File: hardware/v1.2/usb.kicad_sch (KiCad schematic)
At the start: 45 parts, among them J3 USB_C_Receptacle_USB2.0_14P, J4 USB_C_Receptacle_USB2.0_14P, J5 USB_C_Receptacle_USB2.0_14P, U1 ECP5U_25F_CABGA256, U6 FT231XQ, U7 TPD2EUSB30A, U8 TPD2EUSB30A, U9 TPD2EUSB30A

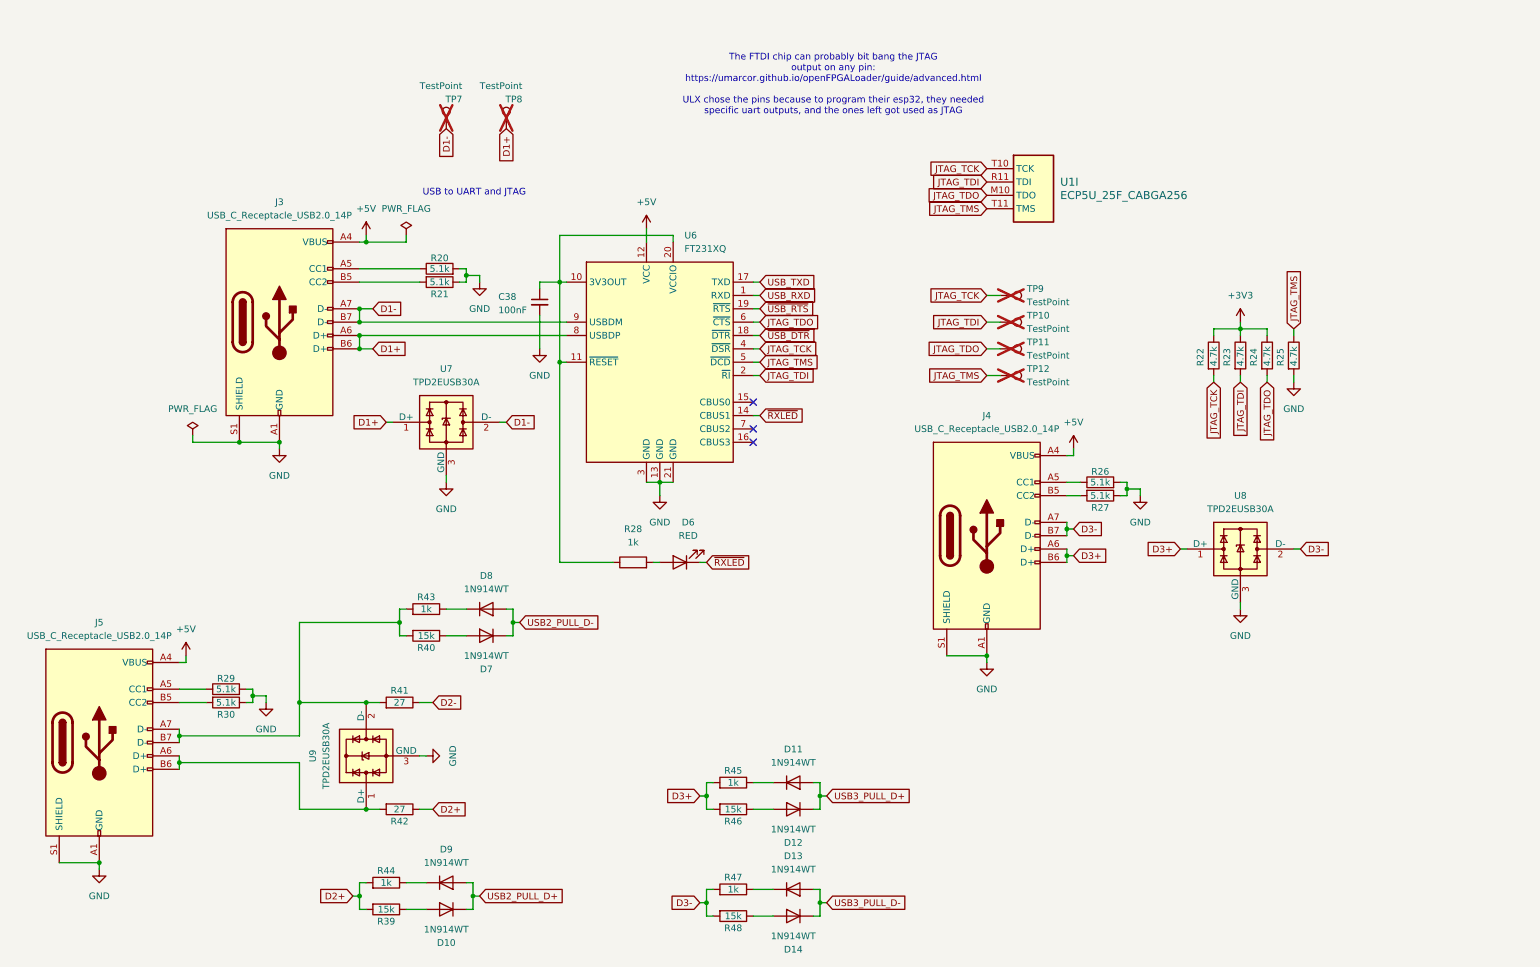
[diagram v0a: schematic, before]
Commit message: Trying to document my journey :)
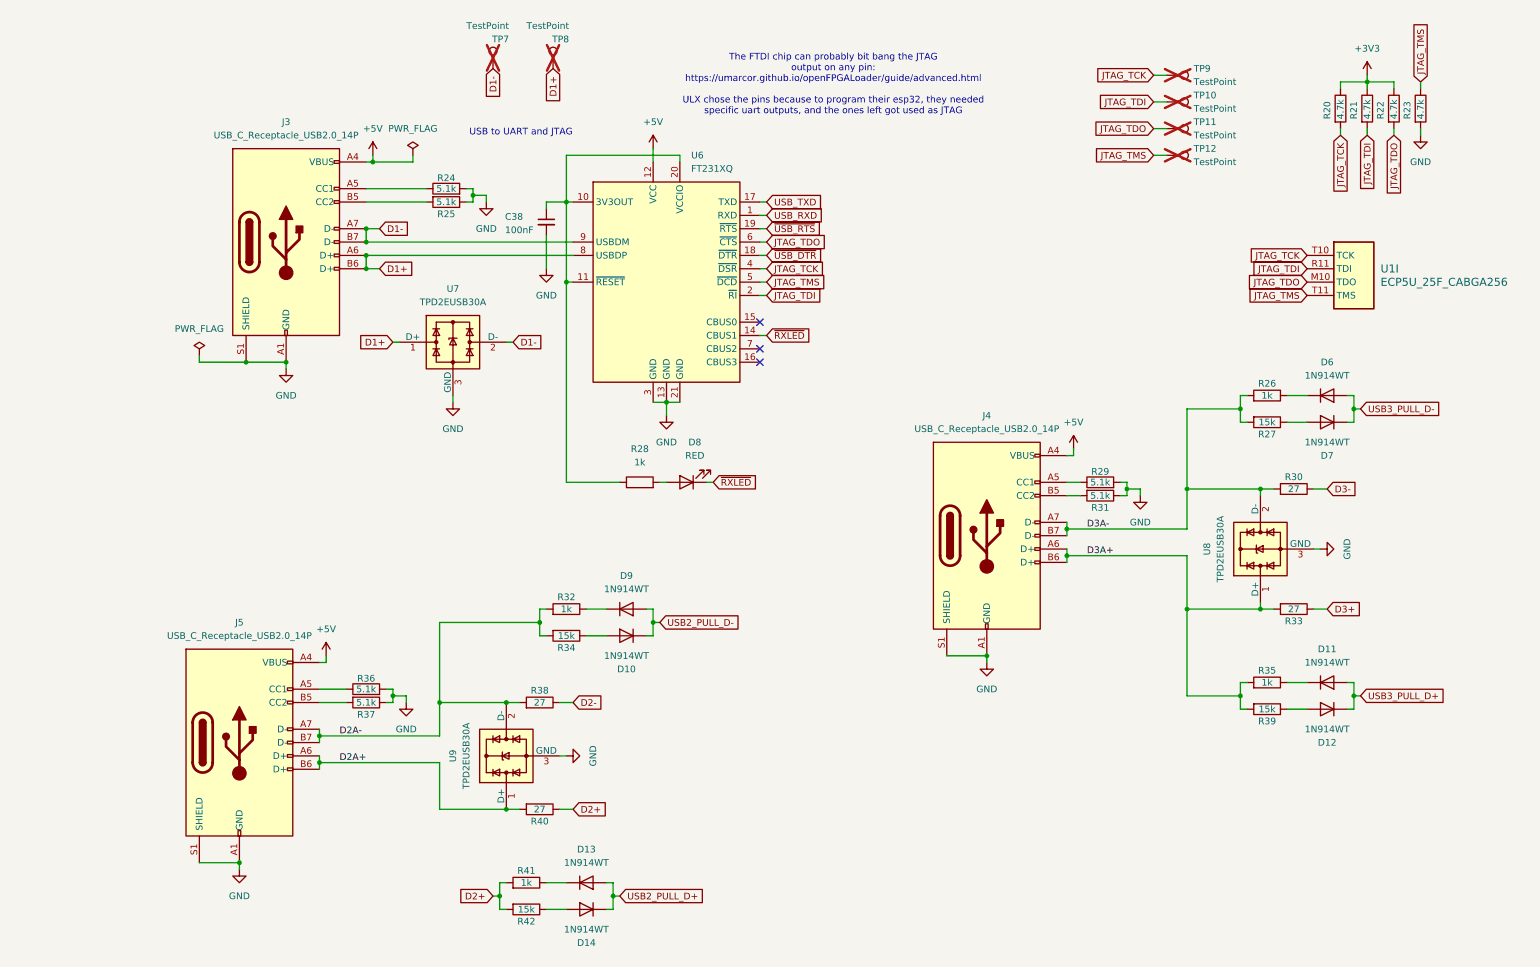
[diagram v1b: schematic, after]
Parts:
- added R30, R33: 27, Resistor_SMD:R_0201_0603Metric, symbol Device:R
- renumbered D7 to D10, D9 to D13, D10 to D14, D13 to D6, D14 to D7, D6 to D8, D8 to D9, R22 to R20, R23 to R21, R24 to R22, R25 to R23, R20 to R24, R21 to R25, R47 to R26, R48 to R27, R26 to R29, R27 to R31, R43 to R32, R40 to R34, R45 to R35, R29 to R36, R30 to R37, R41 to R38, R46 to R39, R42 to R40, R44 to R41, R39 to R42
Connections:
- net D3+: now also R33.1; no longer J4.A6 (D+), J4.B6 (D+), R35.2, R39.2, U8.1 (D+)
- net D3-: now also R30.1; no longer J4.A7 (D-), J4.B7 (D-), R26.2, R27.2, U8.2 (D-)
- net D2A-: now reaches J5.A7 (D-), J5.B7 (D-), R32.2, R34.2, R38.2, U9.2 (D-)
- net D2A+: now reaches J5.A6 (D+), J5.B6 (D+), R40.2, U9.1 (D+)
- new net D3A+: J4.A6 (D+), J4.B6 (D+), R33.2, R35.2, R39.2, U8.1 (D+)
- new net D3A-: J4.A7 (D-), J4.B7 (D-), R26.2, R27.2, R30.2, U8.2 (D-)
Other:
- moved on the sheet: C38, D10, D11, D12, D13, D14, D6, D7, D8, D9, J3, J5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
